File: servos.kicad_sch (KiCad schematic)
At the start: 12 parts, among them J10 171857-0003, J7 171857-0003, J8 171857-0003, J9 171857-0003

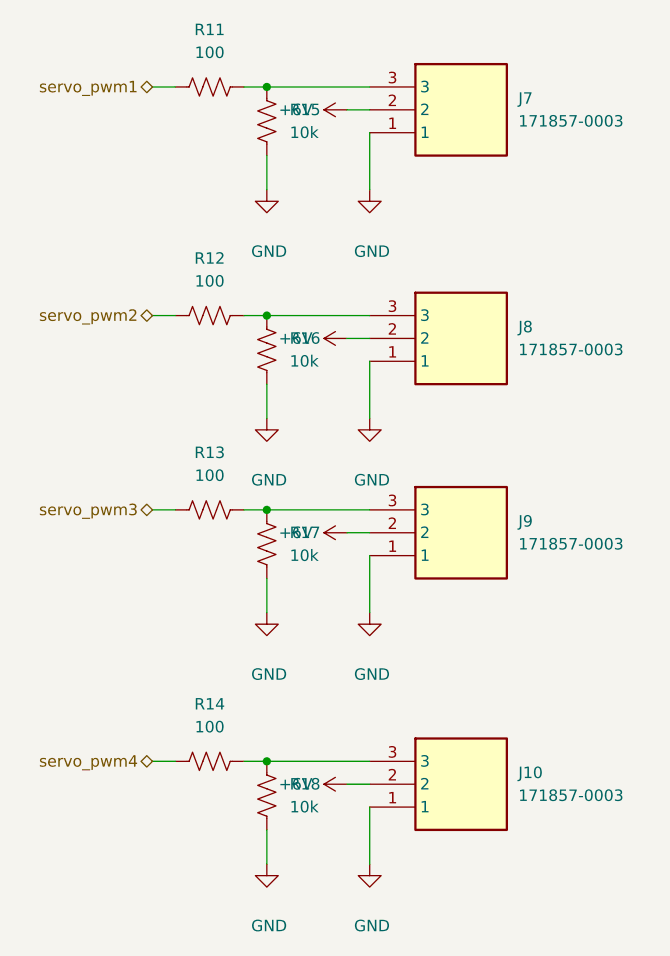
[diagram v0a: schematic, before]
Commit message: sisyphus goes hard, awaiting review.
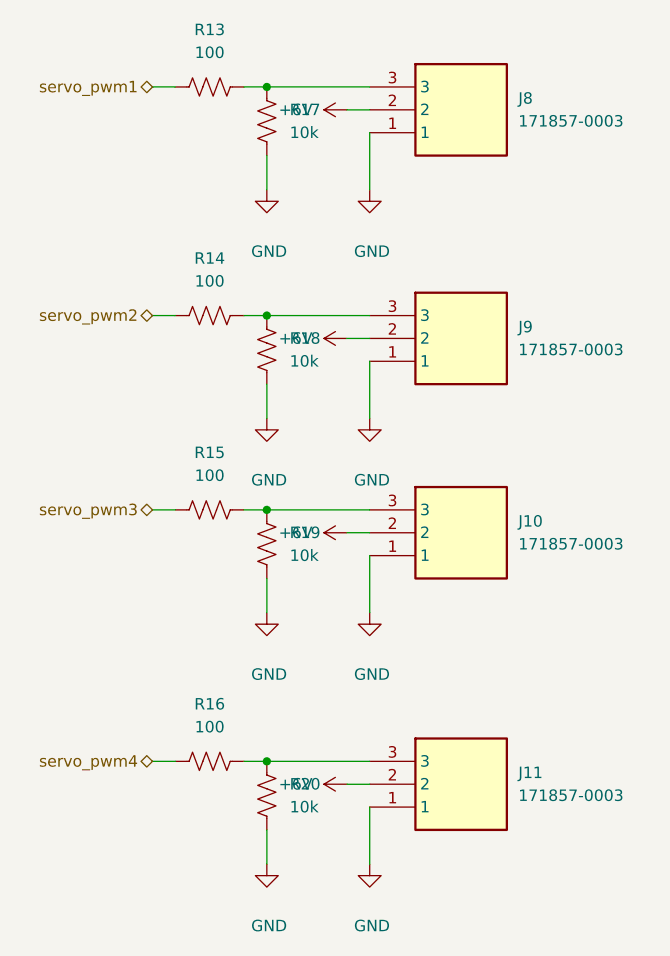
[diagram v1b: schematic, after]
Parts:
- renumbered J9 to J10, J10 to J11, J7 to J8, J8 to J9, R11 to R13, R12 to R14, R13 to R15, R14 to R16, R15 to R17, R16 to R18, R17 to R19, R18 to R20
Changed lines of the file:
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@@
 		(dnp no)
 		(fields_autoplaced yes)
-		(property "Reference" "R14"
+		(property "Reference" "R16"
 			(at 115.57 116.84 0)
 			(show_name no)
@@
 			(project "engineering_plane"
 				(path "/f9a2ded0-d803-4be9-b2f5-4dda0f6b4d9a/a8884140-4da9-49d2-8de3-8d91ee78d46d"
-					(reference "R14")
+					(reference "R16")
 					(unit 1)
 				)
@@
 		(dnp no)
 		(fields_autoplaced yes)
-		(property "Reference" "R13"
+		(property "Reference" "R15"
 			(at 115.57 88.9 0)
 			(show_name no)
@@
 			(project "engineering_plane"
 				(path "/f9a2ded0-d803-4be9-b2f5-4dda0f6b4d9a/a8884140-4da9-49d2-8de3-8d91ee78d46d"
-					(reference "R13")
+					(reference "R15")
 					(unit 1)
 				)
@@
 		(dnp no)
 		(fields_autoplaced yes)
-		(property "Reference" "J7"
+		(property "Reference" "J8"
 			(at 149.86 49.5299 0)
 			(show_name no)
@@
 			(project "engineering_plane"
 				(path "/f9a2ded0-d803-4be9-b2f5-4dda0f6b4d9a/a8884140-4da9-49d2-8de3-8d91ee78d46d"
-					(reference "J7")
+					(reference "J8")
 					(unit 1)
 				)
@@
 		(dnp no)
 		(fields_autoplaced yes)
-		(property "Reference" "J10"
+		(property "Reference" "J11"
 			(at 149.86 124.4599 0)
 			(show_name no)
@@
 			(project "engineering_plane"
 				(path "/f9a2ded0-d803-4be9-b2f5-4dda0f6b4d9a/a8884140-4da9-49d2-8de3-8d91ee78d46d"
-					(reference "J10")
+					(reference "J11")
 					(unit 1)
 				)
@@
 		(dnp no)
 		(fields_autoplaced yes)
-		(property "Reference" "J8"
+		(property "Reference" "J9"
 			(at 149.86 74.9299 0)
 			(show_name no)
@@
 			(project "engineering_plane"
 				(path "/f9a2ded0-d803-4be9-b2f5-4dda0f6b4d9a/a8884140-4da9-49d2-8de3-8d91ee78d46d"
-					(reference "J8")
+					(reference "J9")
 					(unit 1)
 				)
@@
 		(dnp no)
 		(fields_autoplaced yes)
-		(property "Reference" "R11"
+		(property "Reference" "R13"
 			(at 115.57 41.91 0)
 			(show_name no)
@@
 			(project "engineering_plane"
 				(path "/f9a2ded0-d803-4be9-b2f5-4dda0f6b4d9a/a8884140-4da9-49d2-8de3-8d91ee78d46d"
-					(reference "R11")
+					(reference "R13")
 					(unit 1)
 				)
@@
 		(dnp no)
 		(fields_autoplaced yes)
-		(property "Reference" "R15"
+		(property "Reference" "R17"
 			(at 124.46 50.7999 90)
 			(show_name no)
@@
 			(project "engineering_plane"
 				(path "/f9a2ded0-d803-4be9-b2f5-4dda0f6b4d9a/a8884140-4da9-49d2-8de3-8d91ee78d46d"
-					(reference "R15")
+					(reference "R17")
 					(unit 1)
 				)
@@
 		(dnp no)
 		(fields_autoplaced yes)
-		(property "Reference" "R17"
+		(property "Reference" "R19"
 			(at 124.46 97.7899 90)
 			(show_name no)
@@
 			(project "engineering_plane"
 				(path "/f9a2ded0-d803-4be9-b2f5-4dda0f6b4d9a/a8884140-4da9-49d2-8de3-8d91ee78d46d"
-					(reference "R17")
+					(reference "R19")
 					(unit 1)
 				)
@@
 		(dnp no)
 		(fields_autoplaced yes)
-		(property "Reference" "R18"
+		(property "Reference" "R20"
 			(at 124.46 125.7299 90)
 			(show_name no)
@@
 			(project "engineering_plane"
 				(path "/f9a2ded0-d803-4be9-b2f5-4dda0f6b4d9a/a8884140-4da9-49d2-8de3-8d91ee78d46d"
-					(reference "R18")
+					(reference "R20")
 					(unit 1)
 				)
@@
 		(dnp no)
 		(fields_autoplaced yes)
-		(property "Reference" "J9"
+		(property "Reference" "J10"
 			(at 149.86 96.5199 0)
 			(show_name no)
@@
 			(project "engineering_plane"
 				(path "/f9a2ded0-d803-4be9-b2f5-4dda0f6b4d9a/a8884140-4da9-49d2-8de3-8d91ee78d46d"
-					(reference "J9")
+					(reference "J10")
 					(unit 1)
 				)
@@
 		(dnp no)
 		(fields_autoplaced yes)
-		(property "Reference" "R16"
+		(property "Reference" "R18"
 			(at 124.46 76.1999 90)
 			(show_name no)
@@
 			(project "engineering_plane"
 				(path "/f9a2ded0-d803-4be9-b2f5-4dda0f6b4d9a/a8884140-4da9-49d2-8de3-8d91ee78d46d"
-					(reference "R16")
+					(reference "R18")
 					(unit 1)
 				)
@@
 		(dnp no)
 		(fields_autoplaced yes)
-		(property "Reference" "R12"
+		(property "Reference" "R14"
 			(at 115.57 67.31 0)
 			(show_name no)
@@
 			(project "engineering_plane"
 				(path "/f9a2ded0-d803-4be9-b2f5-4dda0f6b4d9a/a8884140-4da9-49d2-8de3-8d91ee78d46d"
-					(reference "R12")
-					(unit 1)
-				)
+					(reference "R14")
+					(unit 1)
+				)
